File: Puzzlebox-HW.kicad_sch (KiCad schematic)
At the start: 8 parts, among them M1 Mount_M3, M2 Mount_M3, M3 Mount_M3, M4 Mount_M3

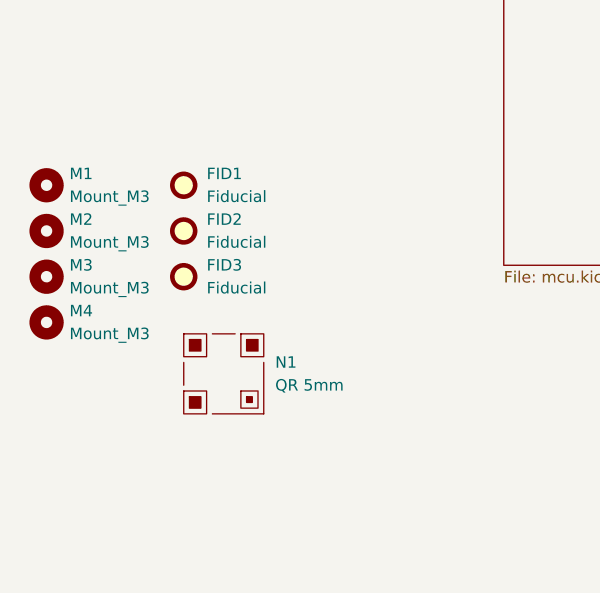
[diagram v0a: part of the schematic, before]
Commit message: Initial layout
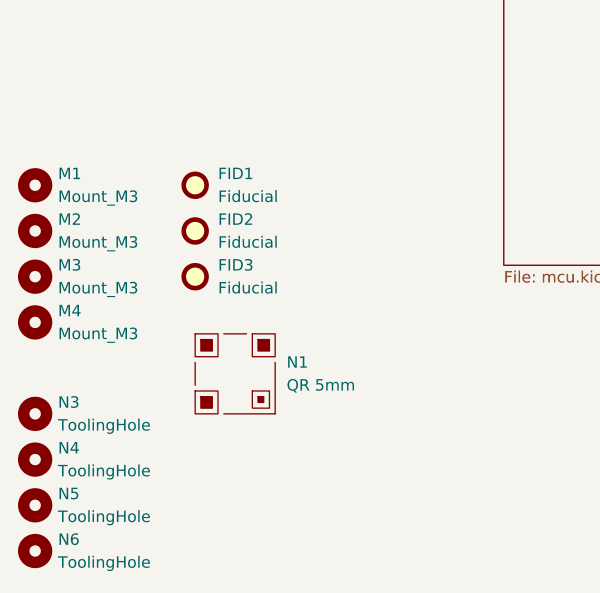
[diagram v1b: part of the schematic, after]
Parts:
- added N3, N4, N5, N6: ToolingHole, N_NonPart:ToolingHole_1mm, symbol N_NonPart:ToolingHole_1mm
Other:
- moved on the sheet: FID1, FID2, FID3, M1, M2, M3, M4, N1
